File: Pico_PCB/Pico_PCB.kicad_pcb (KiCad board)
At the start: 2 copper layers, 60.1 x 41.9 mm, 73 parts, among them J1 USB_A, J4 Conn_02x04_Counter_Clockwise, SW1 SPST_Momentary_4.6x2.8mm, SW2 SPST_Momentary_4.6x2.8mm, U1 AT90USB647-A, Y1 Crystal_GND24

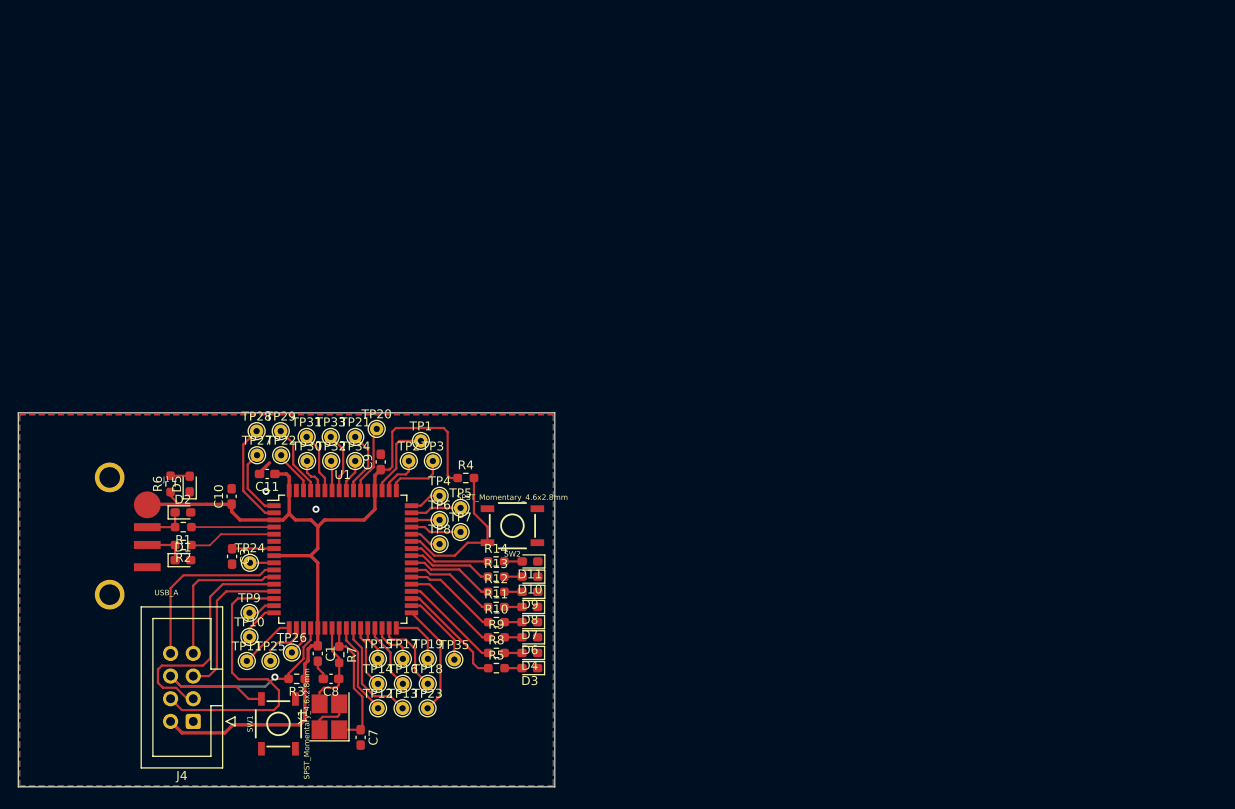
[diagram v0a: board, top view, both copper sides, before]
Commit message: PCB_fini
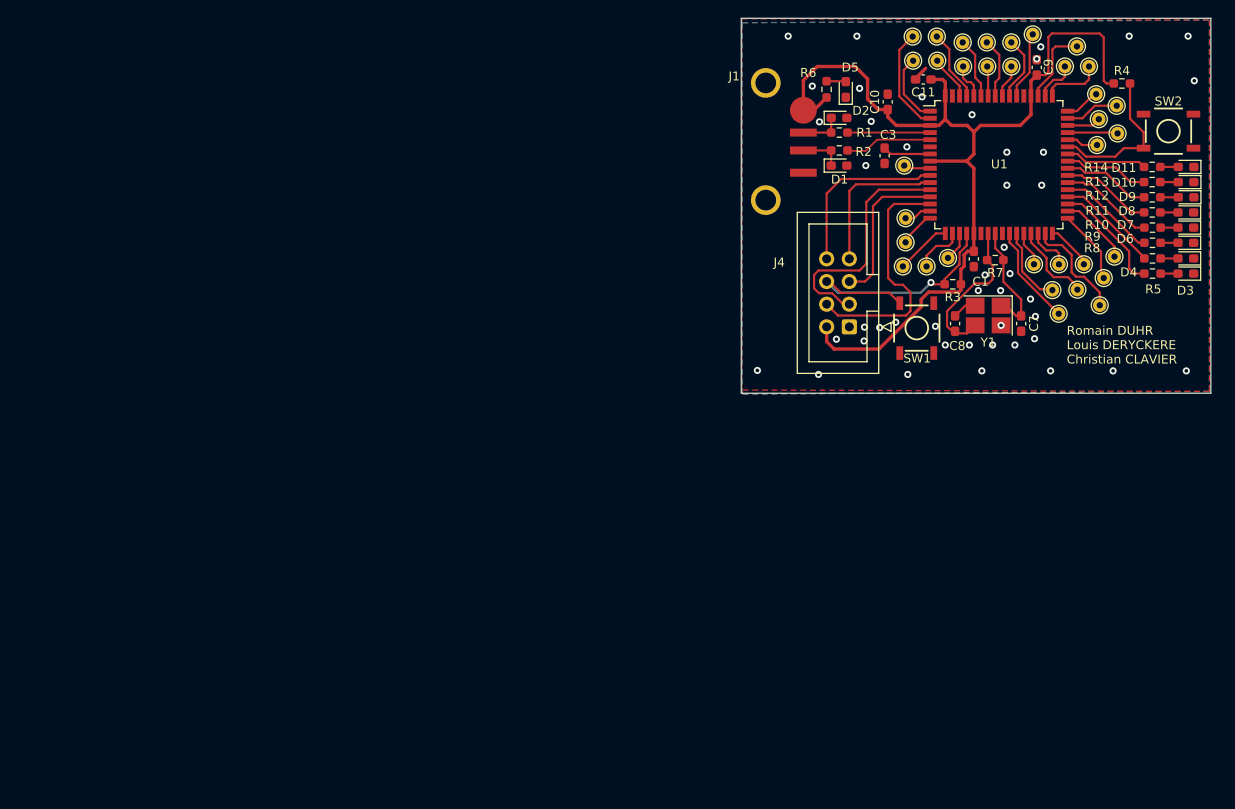
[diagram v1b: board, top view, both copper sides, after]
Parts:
- removed TP12: TestPoint, TestPoint:TestPoint_THTPad_D1.5mm_Drill0.7mm
- C1: value 4.7 uF -> 1uF
- C10: value 100nF -> 1uF
- C11: value 4.7 uF -> 100nF
- C9: value 4.7uF -> 100nF
- moved TP23 89.8 mm to (271.1, 43.7)
- moved TP16 87.5 mm to (268.1, 45.0)
- moved TP14 87.5 mm to (265.3, 45.0)
- moved C7 87.3 mm to (261.8, 48.8)
- moved TP35 86.6 mm to (272.2, 41.3)
- moved TP6 86.4 mm to (270.5, 25.9)
- moved Y1 86.4 mm to (258.1, 47.9), turned to 180 degrees
- moved TP18 86.4 mm to (270.6, 46.8)
- moved TP4 86.2 mm to (270.2, 23.1)
- moved TP5 86.2 mm to (272.5, 24.4)
- moved TP8 86.2 mm to (270.3, 28.8)
- moved TP7 86.1 mm to (272.6, 27.5)
- moved C3 85.8 mm to (246.5, 30.0)
- moved R13 85.8 mm to (276.5, 33.0)
- moved R14 85.8 mm to (276.5, 31.2)
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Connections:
- U1 pad 25: Net-(U1-PD0) -> unconnected-(U1-PD0-Pad25)
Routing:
- net Net-(U1-PD0): track 10.5 -> 0.00 mm
- net +5V: track 102.4 -> 111.3 mm
- net Net-(U1-XTAL2): track 10.5 -> 17.6 mm
- net INT: track 33.2 -> 28.0 mm
- net Net-(U1-PE0): track 12.6 -> 8.38 mm
- net GND: track 8.73 -> 4.53 mm, vias 2 -> 45
- net Net-(U1-PD6): track 8.95 -> 12.0 mm
- net Net-(U1-XTAL1): track 15.4 -> 13.4 mm
- net RESET: track 32.2 -> 30.2 mm
- net Net-(U1-PD4): track 7.55 -> 9.39 mm
- net Net-(U1-PD1): track 12.3 -> 11.3 mm
- net Net-(U1-PD7): track 6.30 -> 5.27 mm
- net Net-(U1-PD2): track 7.06 -> 7.94 mm
- net 3.3V: track 4.71 -> 5.37 mm
- net Net-(U1-PA5): track 3.15 -> 3.79 mm
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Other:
- board size 60.1 x 41.9 mm -> 52.6 x 42 mm
- board text added: "Romain DUHR Louis DERYCKERE Christian CLAVIER"
